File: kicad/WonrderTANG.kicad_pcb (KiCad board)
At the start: 2 copper layers, 101.6 x 90.2 mm, 33 parts, among them CON1 MSX-CONNECTOR, J1 Conn_02x01, J2 AudioJack3, J3 Conn_02x01, Q1 2N3904, Q2 2N3904, U1 SN74LVC245AN, U2 SN74LVC245AN, U3 SN74LVC245AN, U4 SN74LVC245AN, U5 Tang_Nano_20k, U6 SN74LVC245AN

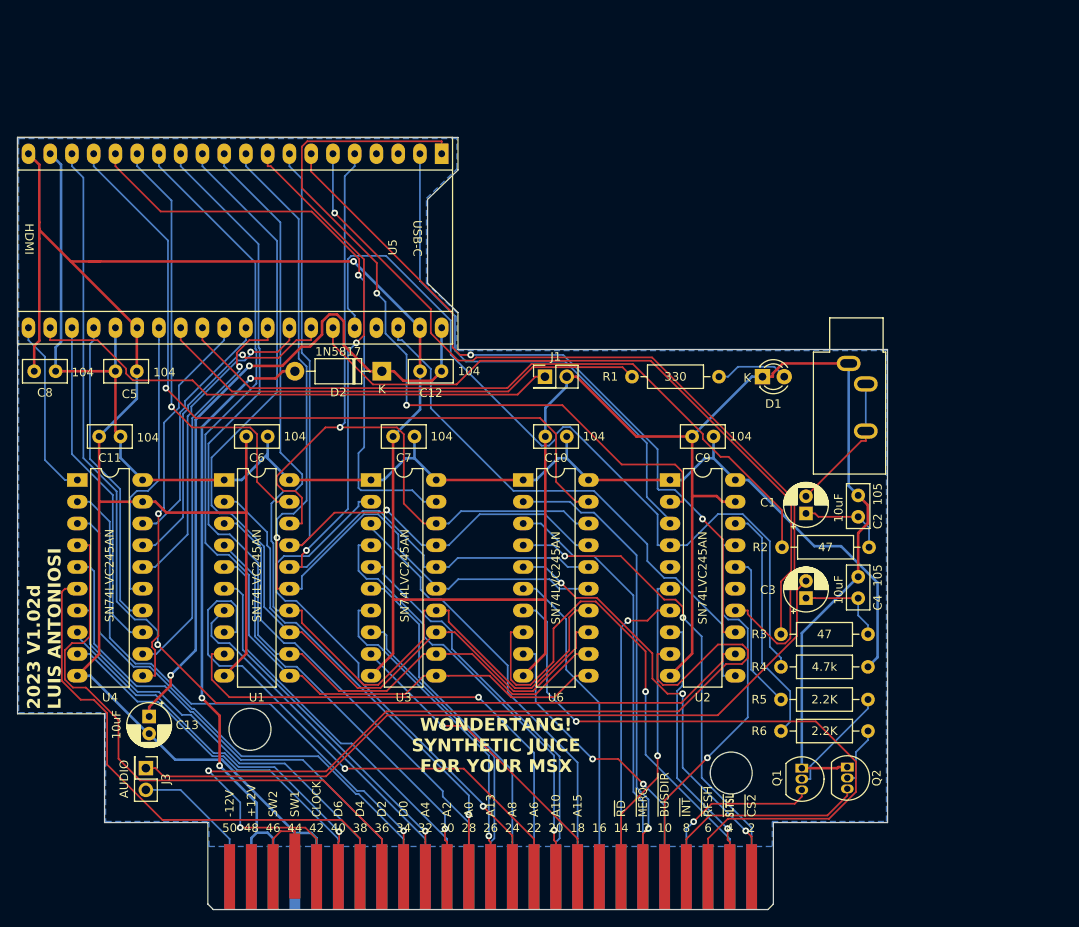
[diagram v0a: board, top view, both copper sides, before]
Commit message: version 2.0b
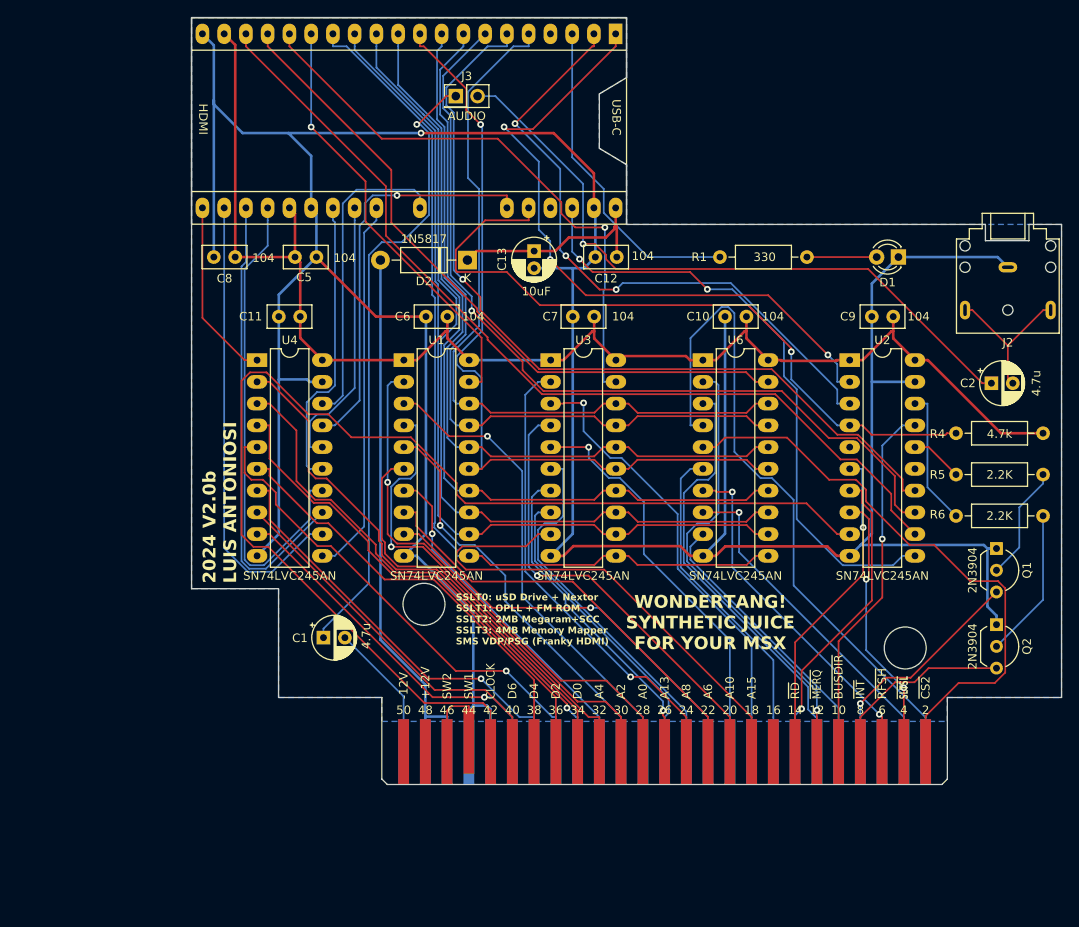
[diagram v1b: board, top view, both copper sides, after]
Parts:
- removed C3: 10uF, Capacitor_THT:CP_Radial_D5.0mm_P2.00mm
- removed C4: 105, Capacitor_THT:C_Disc_D5.0mm_W2.5mm_P2.50mm
- removed J1: Conn_02x01, Connector_PinHeader_2.54mm:PinHeader_2x01_P2.54mm_Vertical
- removed R2, R3: 47, Resistor_THT:R_Axial_DIN0207_L6.3mm_D2.5mm_P10.16mm_Horizontal
- C1: value 10uF -> 4.7u; footprint Capacitor_THT:CP_Radial_D5.0mm_P2.00mm -> Capacitor_THT:CP_Radial_D5.0mm_P2.50mm
- C2: value 105 -> 4.7u; footprint Capacitor_THT:C_Disc_D5.0mm_W2.5mm_P2.50mm -> Capacitor_THT:CP_Radial_D5.0mm_P2.50mm
- CON1: footprint Mis_huellas:CARTRIDGE_MSX -> Tang20K:CARTRIDGE_MSX_NOCUT
- D1: value LED -> uSD
- J2: footprint Connector_Audio:Jack_3.5mm_CUI_SJ1-3533NG_Horizontal -> Tang20K:SJ1-3523N
- J3: value Conn_02x01 -> AUDIO
- Q1, Q2: footprint Package_TO_SOT_THT:TO-92_Inline -> Package_TO_SOT_THT:TO-92_Inline_Wide
- U5: footprint Mis_huellas:Tang_Nano_20k -> Tang20K:Tang_Nano_20k_Audio
- moved J3 86.4 mm to (107.7, 48.5), turned to 0 degrees
- moved C13 70.5 mm to (116.8, 66.6)
- moved C1 58.2 mm to (92.2, 111.8), turned to 0 degrees
- moved Q1 34.3 mm to (170.8, 101.3)
- moved R4 34.1 mm to (176.3, 87.9)
- moved R5 33.3 mm to (166.1, 92.7)
- moved R6 32.4 mm to (166.1, 97.5)
- moved C9 25.2 mm to (158.8, 74.3)
- moved U6 25.2 mm to (136.6, 79.3)
- moved C11 25.2 mm to (89.5, 74.3)
- moved C6 25.2 mm to (106.7, 74.3)
- moved C7 25.2 mm to (123.9, 74.3)
- moved U1 25.2 mm to (101.6, 79.3)
- moved U3 25.2 mm to (118.8, 79.3)
- moved U4 25.2 mm to (84.5, 79.3)
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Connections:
- C1 pad 1: Net-(C1-Pad1) -> Net-(J3-Pin_1)
- C1 pad 2: Net-(C1-Pad2) -> SOUNDIN
- C2 pad 1: Net-(C1-Pad1) -> Net-(J3-Pin_2)
- C2 pad 2: GND -> Net-(C2-Pad2)
- J2 pad R: Net-(C1-Pad2) -> Net-(C2-Pad2)
- J2 pad T: Net-(C1-Pad2) -> Net-(C2-Pad2)
- J3 pad 2: SOUNDIN -> Net-(J3-Pin_2)
- U5 pad 22: JP -> D6_33
- U5 pad 28: LED -> D2_33
- U5 pad 29: SOUND_33 -> D7_33
- U5 pad 3: unconnected-(U5-75_IOT34A-Pad3) -> LED
- U5 pad 35: AUDIO_33 -> D1_33
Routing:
- net SOUND_33: track 84.4 -> 0.00 mm
- net AUDIO_33: track 81.4 -> 0.00 mm
- net Net-(J3-Pin_2): track 0.00 -> 78.3 mm, vias 0 -> 1
- net JP: track 63.1 -> 0.00 mm
- net +5V: track 82.0 -> 24.9 mm, vias 2 -> 0
- net GND: track 451.9 -> 412.2 mm
- net RFSH: track 78.5 -> 41.1 mm, vias 1 -> 2
- net CLOCK: track 109.0 -> 140.5 mm, vias 2 -> 0
- net SLTSL_33: track 135.4 -> 107.9 mm, vias 1 -> 0
- net CS1: track 56.5 -> 79.9 mm, vias 2 -> 0
- net CS12: track 62.1 -> 40.2 mm
- net A15: track 37.6 -> 58.9 mm, vias 1 -> 0
- net MP4_33: track 116.6 -> 95.8 mm
- net D4_33: track 36.6 -> 57.1 mm
- net LED: track 58.3 -> 38.1 mm
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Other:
- board size 101.6 x 90.2 mm -> 101.6 x 89.5 mm
- board text added: "2024 V2.0b LUIS ANTONIOSI"
- board text added: "SSLT0: uSD Drive + Nextor SSLT1: OPLL + FM ROM SSLT2: 2MB Megaram+SCC SSLT3: 4MB Memory Mapper SMS VDP/PSG (Franky HDMI)"
- board text removed: "2023 V1.02d LUIS ANTONIOSI"
